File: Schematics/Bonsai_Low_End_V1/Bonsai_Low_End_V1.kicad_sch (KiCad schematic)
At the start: 19 parts, among them U1 MOUDLE-SEEEDUINO-XIAO-ESP32C3, U2 MAX30101EFD, U3 RE1C002UN, U4 RE1C002UN, U5 DRV2605LDGS

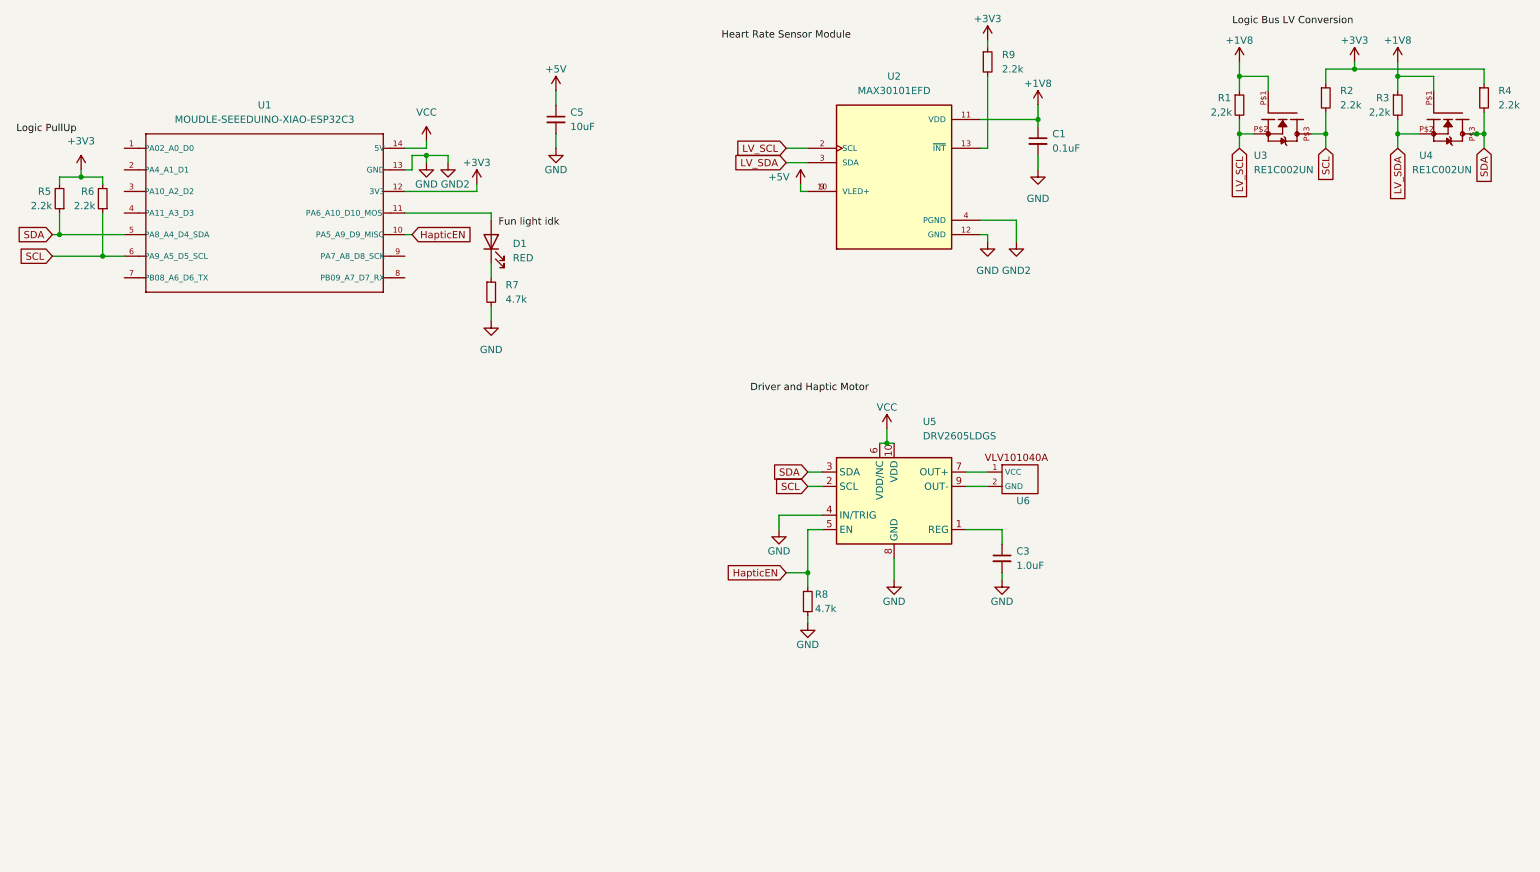
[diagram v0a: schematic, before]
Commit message: last psuh before feedback
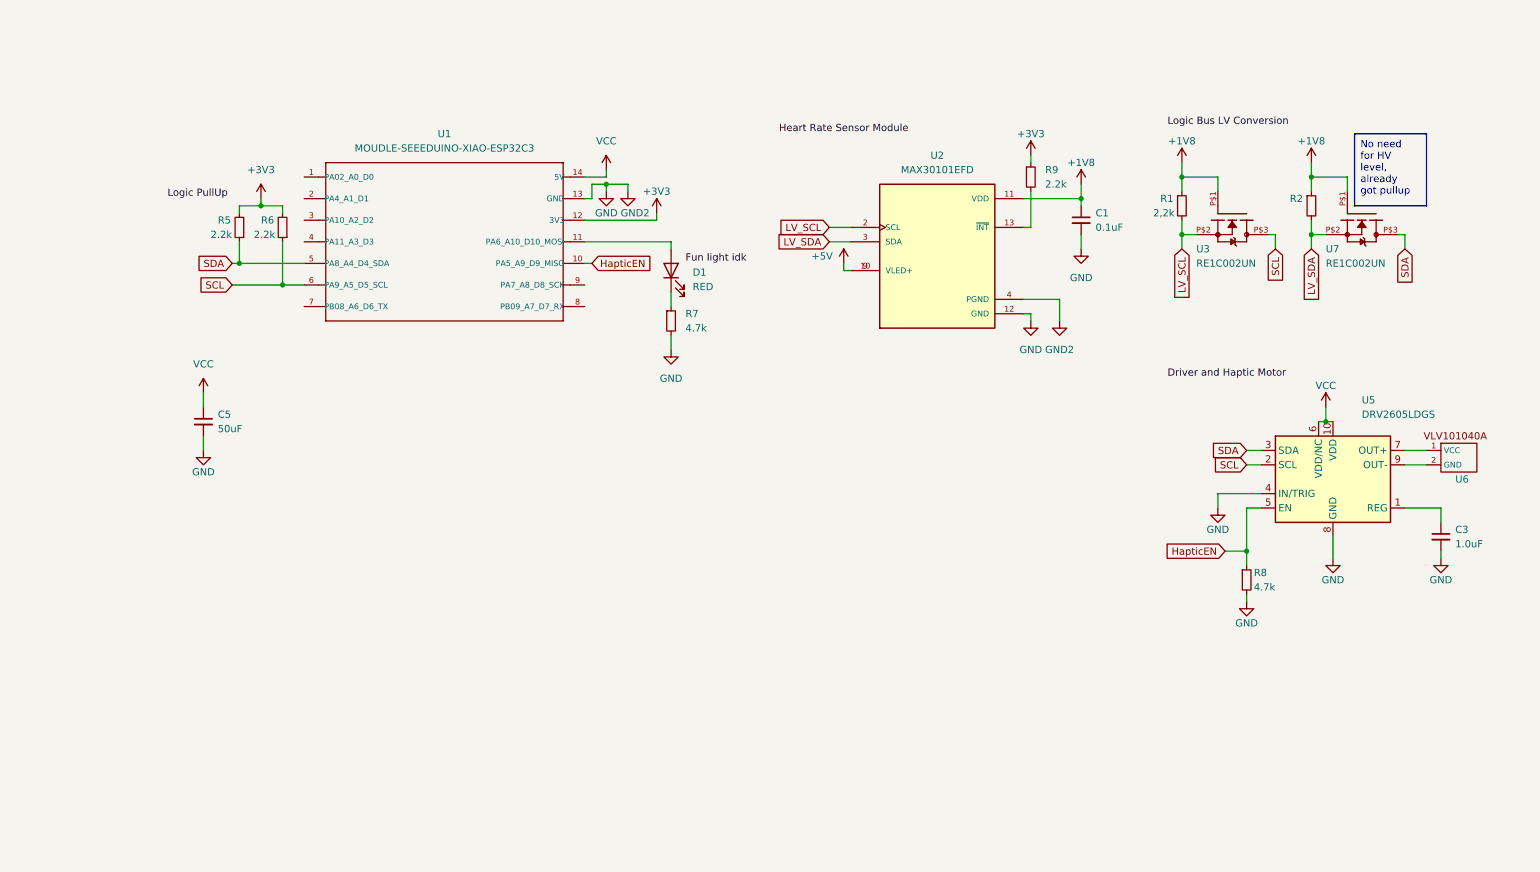
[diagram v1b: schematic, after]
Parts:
- removed R3: 2,2k, symbol Device:R_Small
- removed R4: 2.2k, symbol Device:R_Small
- removed U4: RE1C002UN, RE1C002UN:EMT3F, symbol RE1C002UN:RE1C002UN
- added U7: RE1C002UN, RE1C002UN:EMT3F, symbol RE1C002UN:RE1C002UN
- C5: value 10uF -> 50uF
- R2: value 2.2k -> 2,2k
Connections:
- net +1V8: now also R2.1, U7.P$1
- net +3V3: no longer R2.1
- net +5V: no longer C5.1
- net LV_SDA: now also R2.2, U7.P$2
- net SCL: no longer R2.2
- net SDA: now also U7.P$3
- net VCC: now also C5.1
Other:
- company: (none) -> Bonsai
- title: (none) -> Bonsai Wearable Prototype
- moved on the sheet: C1, C3, C5, D1, R1, R5, R6, R7, R8, R9, U1, U2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

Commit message: Made PCB
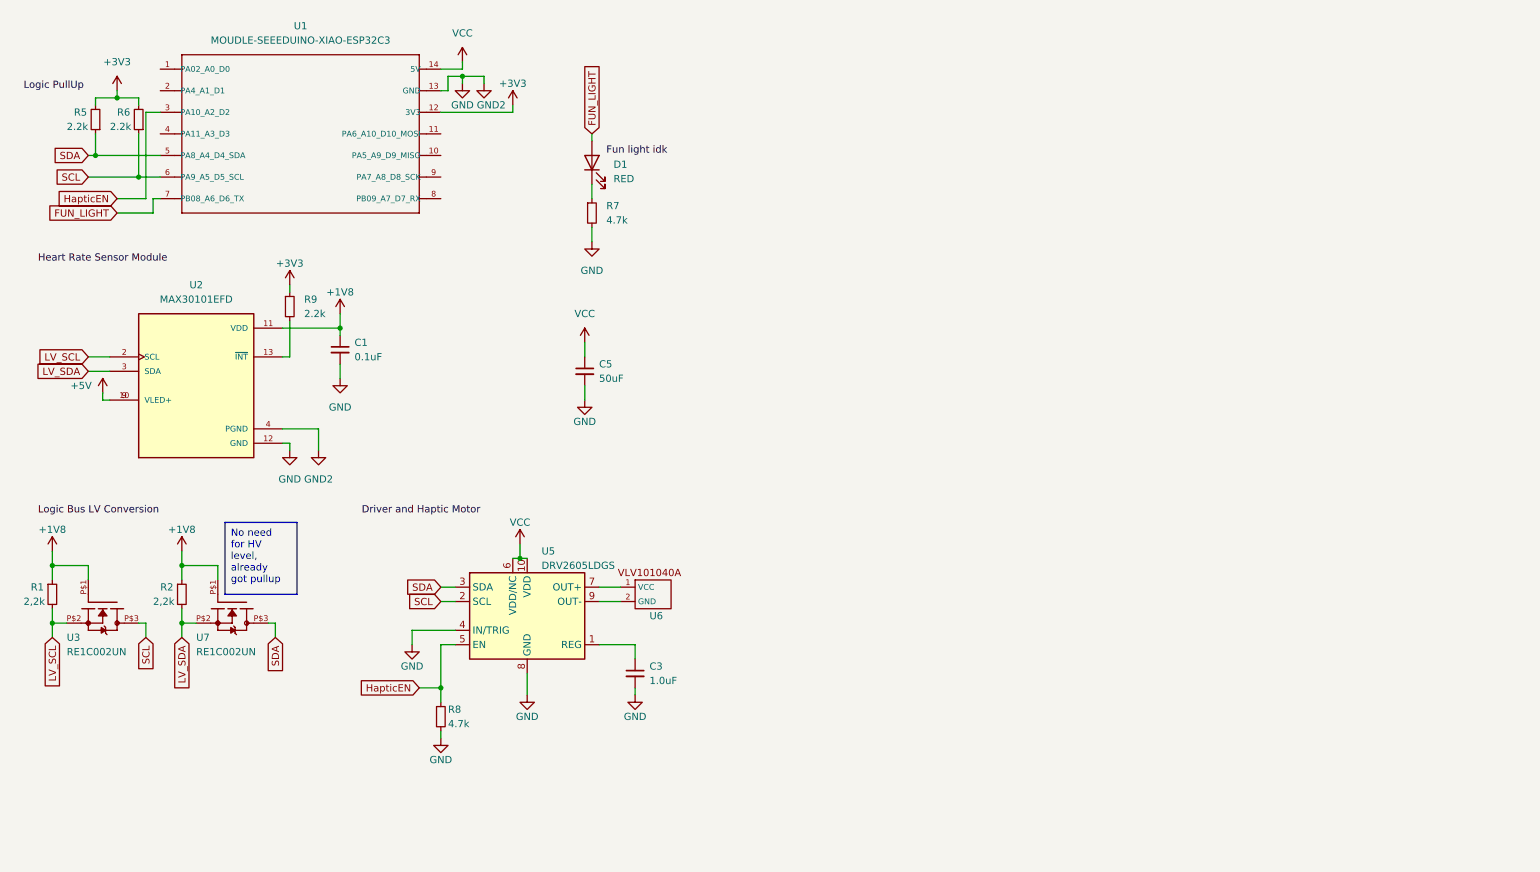
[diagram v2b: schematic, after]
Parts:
- C1, C3: footprint (none) -> Capacitor_SMD:C_0603_1608Metric_Pad1.08x0.95mm_HandSolder
- C5: footprint (none) -> Capacitor_SMD:C_0805_2012Metric_Pad1.18x1.45mm_HandSolder
- D1: footprint (none) -> LED_SMD:LED_0603_1608Metric_Pad1.05x0.95mm_HandSolder
- R1, R2, R5, R6, R7, R8, R9: footprint (none) -> Resistor_SMD:R_0603_1608Metric_Pad0.98x0.95mm_HandSolder
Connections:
- net HapticEN: now also U1.3 (PA10_A2_D2); no longer U1.10 (PA5_A9_D9_MISO)
- net at U1.11 (PA6_A10_D10_MOSI): no longer D1.2 (A)
- net FUN_LIGHT: now reaches U1.7 (PB08_A6_D6_TX)
- net FUN_LIGHT: now also D1.2 (A)
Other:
- moved on the sheet: C1, C3, C5, D1, R1, R2, R5, R6, R7, R8, R9, U1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

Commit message: Improved
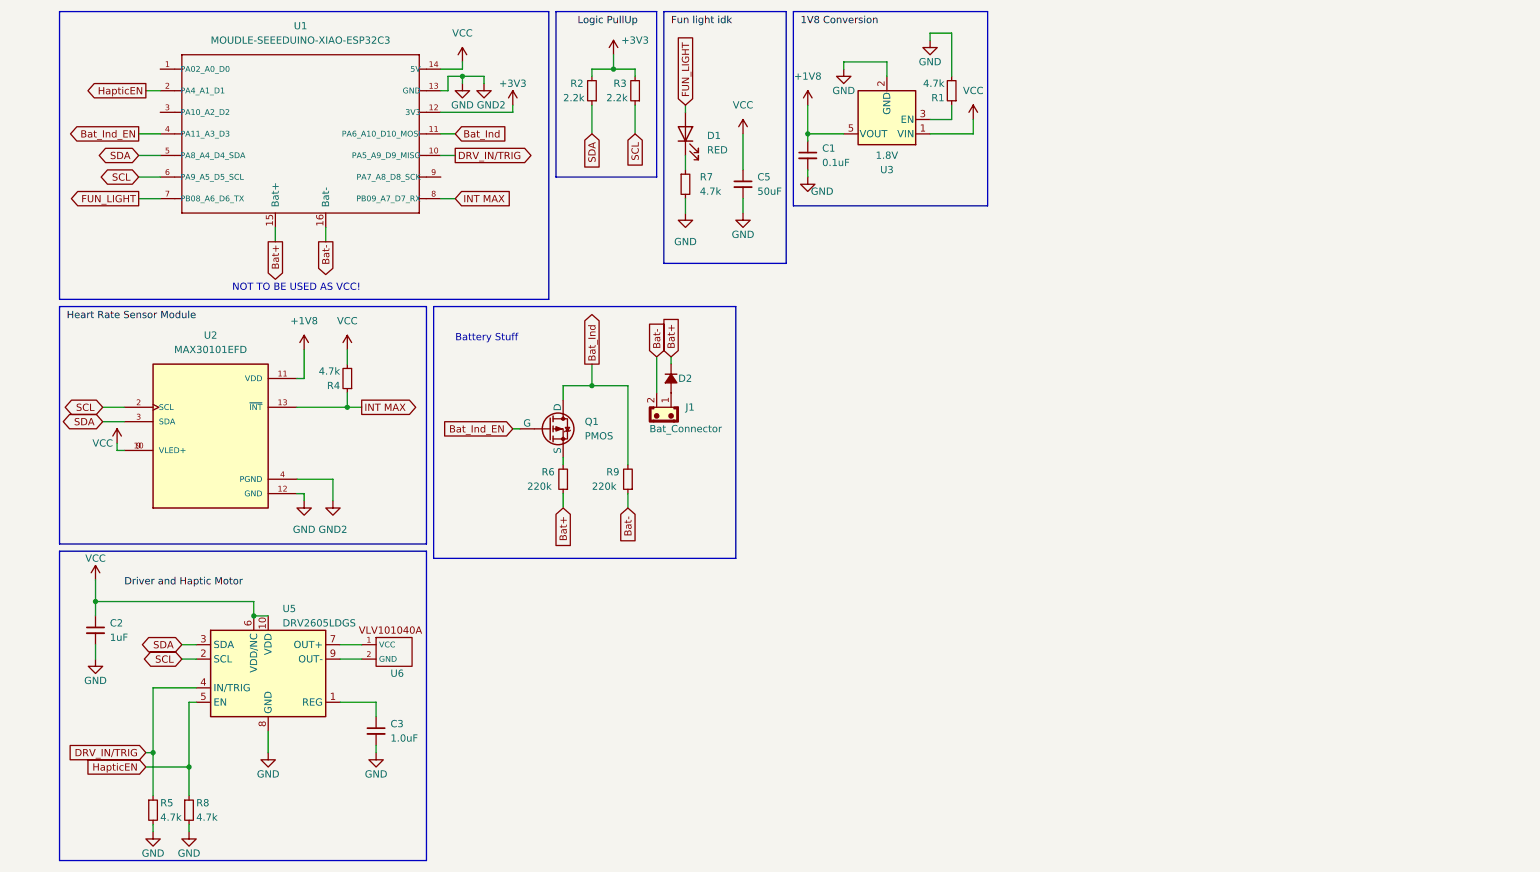
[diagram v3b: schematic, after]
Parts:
- removed U3, U7: RE1C002UN, RE1C002UN:EMT3F, symbol RE1C002UN:RE1C002UN
- added C2: 1uF, Capacitor_SMD:C_0805_2012Metric_Pad1.18x1.45mm_HandSolder, symbol Device:C_Small
- added D2: D_Small_Filled, symbol Device:D_Small_Filled
- added J1: Bat_Connector, Connector_JST:JST_EH_B2B-EH-A_1x02_P2.50mm_Vertical, symbol PCM_SL_Connectors:JST_02
- added Q1: PMOS, symbol Simulation_SPICE:PMOS
- added R3: 2.2k, Resistor_SMD:R_0603_1608Metric_Pad0.98x0.95mm_HandSolder, symbol Device:R_Small
- added R4: 4.7k, Resistor_SMD:R_0603_1608Metric_Pad0.98x0.95mm_HandSolder, symbol Device:R_Small
- added U3: 1.8V, Package_TO_SOT_SMD:SOT-23-5, symbol Regulator_Linear:AP2204K-1.8
- R1: value 2,2k -> 4.7k
- R2: value 2,2k -> 2.2k
- R5: value 2.2k -> 4.7k
- R6, R9: value 2.2k -> 220k
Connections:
- net +5V is gone; now on net VCC: U2.10 (VLED+), U2.9 (VLED+)
- net +1V8: now also U3.5 (VOUT); no longer R1.1, R2.1
- net +3V3: now also R2.2, R3.2; no longer R5.2, R6.2, R9.1
- net GND: now also R1.2, R5.2, C2.2, U3.2 (GND); no longer U5.4 (IN/TRIG)
- net HapticEN: now also U1.2 (PA4_A1_D1); no longer U1.3 (PA10_A2_D2)
- net SCL: now also U2.2 (SCL), R3.1; no longer R6.1
- net SDA: now also R2.1, U2.3 (SDA); no longer R5.1
- net VCC: now also C2.1, R4.2, U3.1 (VIN)
- net Bat_Ind: now reaches R9.2
- net Bat_Ind: now also U1.11 (PA6_A10_D10_MOSI), Q1.1 (D); no longer U2.13 (~{INT})
- net DRV_IN/TRIG: now reaches U1.10 (PA5_A9_D9_MISO)
- net DRV_IN/TRIG: now also R5.1, U5.4 (IN/TRIG)
- net Bat_Ind_EN: now reaches U1.4 (PA11_A3_D3)
- net Bat_Ind_EN: now also Q1.2 (G)
- net INT MAX: now reaches U1.8 (PB09_A7_D7_RX)
- net INT MAX: now also U2.13 (~{INT}), R4.1
- removed net LV_SCL: R1.2, U2.2 (SCL)
- removed net LV_SDA: R2.2, U2.3 (SDA)
- new net: Q1.3 (S), R6.2
- new net: R1.1, U3.3 (EN)
- new net: D2.2 (A), J1.1
- new net Bat+: D2.1 (K), R6.1, U1.15 (Bat+)
- new net Bat-: J1.2, R9.1, U1.16 (Bat-)
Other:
- note added: "Battery Stuff"
- note added: "NOT TO BE USED AS VCC!"
- moved on the sheet: C3, C5, D1, R7, R8, U2, U5, U6
